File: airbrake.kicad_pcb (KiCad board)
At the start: 2 copper layers, 53.8 x 52.2 mm, 81 parts, among them IC1 SN74HCT125DR, J1 Molex Microfit, J2 Molex Microfit, J3 Molex Microfit, J4 Molex Microfit, J5 Molex Microfit, J6 Conn_02x03_Counter_Clockwise, U1 MS5607-02BA, U2 MMC5983MA, U3 STM32G431RBTx, U4 TMP275AIDGKR VSSOP8, U5 LP5912Q3.3DRVRQ1, U6 BMI088, U7 TPS62153, U8 USBLC6-2SC6, U9 W25Q256JVEIQTR, X1 1XXD32000MBA

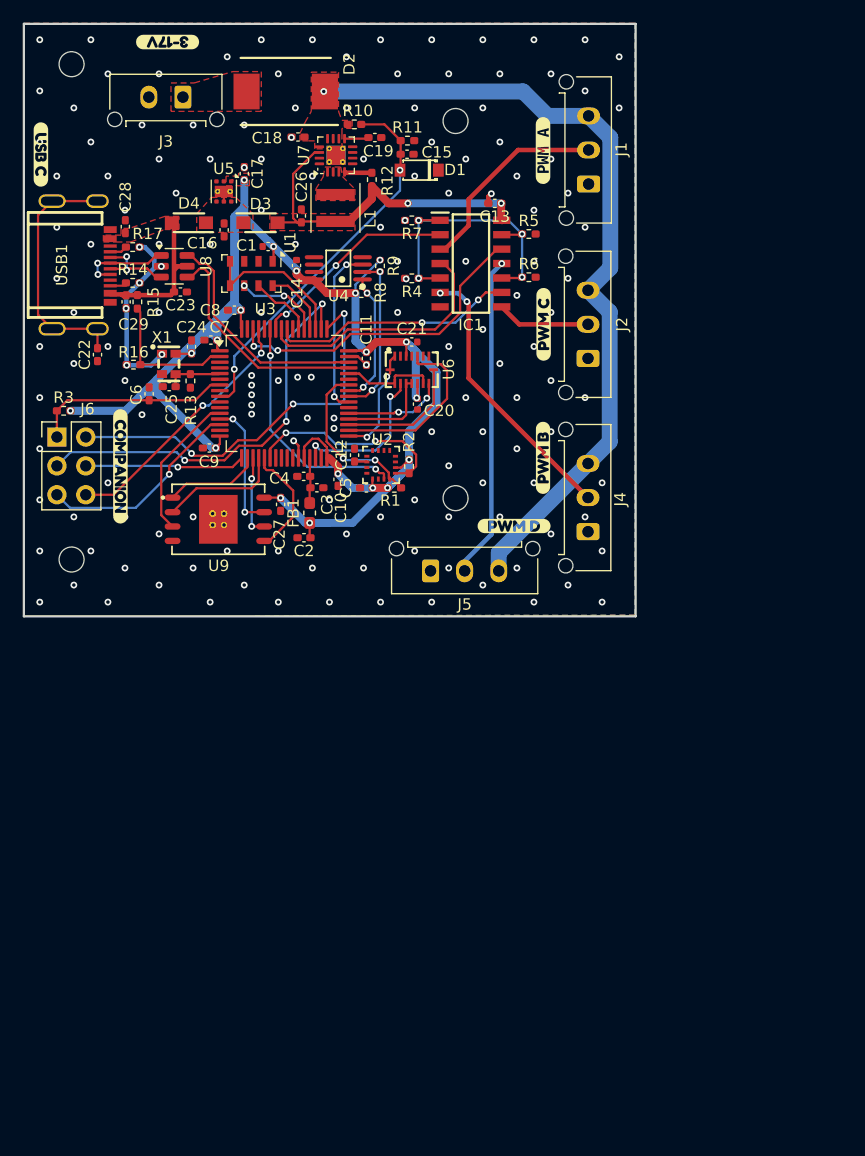
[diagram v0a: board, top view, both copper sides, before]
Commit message: release: rev1
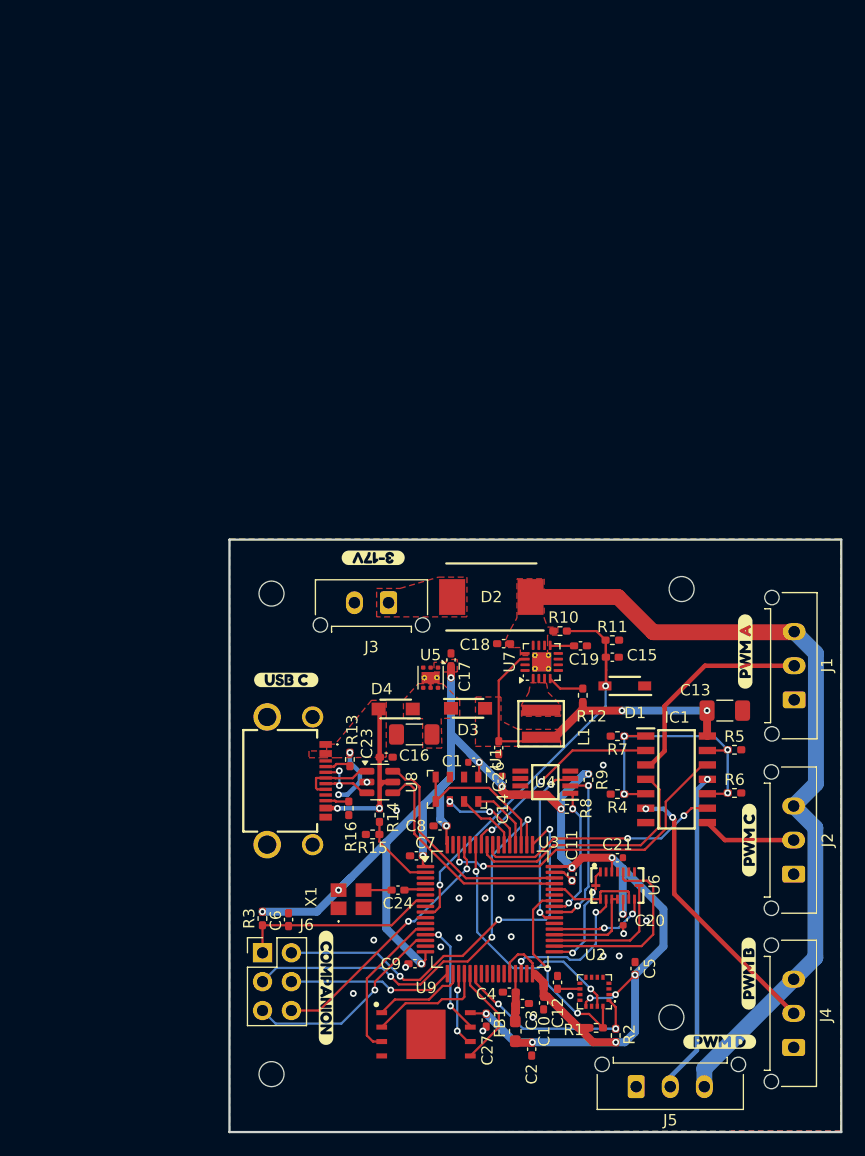
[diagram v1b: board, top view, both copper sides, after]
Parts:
- removed C22: 1nF, Capacitor_SMD:C_0402_1005Metric_Pad0.74x0.62mm_HandSolder
- removed C25: 10pF, Capacitor_SMD:C_0402_1005Metric_Pad0.74x0.62mm_HandSolder
- removed C28, C29: 10uF, Capacitor_SMD:C_0402_1005Metric_Pad0.74x0.62mm_HandSolder
- removed R17: 5.1k, Resistor_SMD:R_0402_1005Metric_Pad0.72x0.64mm_HandSolder
- removed kibuzzard-67AC9DAB: G***, kibuzzard-67AC9DAB
- added kibuzzard-67B37024: G***, kibuzzard-67B37024, F.Cu at (169.1, 89.3)
- C13, C16: footprint Capacitor_SMD:C_0402_1005Metric_Pad0.74x0.62mm_HandSolder -> Capacitor_SMD:C_1206_3216Metric_Pad1.33x1.80mm_HandSolder
- C24: value 100nF -> 10nF
- D1: footprint EasyEDA:SOD-123_L2.8-W1.8-LS3.7-RD -> SamacSys:SOD3716X135N
- D2: footprint Samacsys:DIOM7959X262N -> SamacSys:DIOM7959X262N
- D3, D4: footprint Samacsys:SODFL3616X98N -> SamacSys:SODFL3616X98N
- IC1: footprint Samacsys:SOIC127P600X175-14N -> SamacSys:SOIC127P600X175-14N
- L1: footprint Inductor_SMD:L_Coilcraft_XxL4020 -> SamacSys:XFL4020472MEC
- R13: value 100k -> 5.1k
- R14: value 5.1k -> 10k
- R15: value 10k -> 22k
- R16: value 22k -> 5.1k
- U1: value MS5607-02BA -> MS560702BA03-50
- U2: footprint EasyEDA:LGA-16_L3.0-W3.0-P0.50-BL_SQ -> SamacSys:MMC5983MA
- U4: value TMP275AIDGKR VSSOP8 -> TMP275AIDGKR; footprint EasyEDA:VSSOP-8_L3.0-W3.0-P0.65-LS5.0-BL -> SamacSys:SOP65P490X110-8N
- U9: footprint EasyEDA:WSON-8_L8.0-W6.10-P1.27-BL-EP -> SamacSys:SON127P800X600X80-9N-D
- USB1: value C169130 -> 10172013-00011LF; footprint EasyEDA:USB-C-SMD_TYPE-C3.1-02 -> SamacSys:1017201300011LF
- X1: value 1XXD32000MBA -> ECS-TXO-32CSMV-320-AN-TR; footprint EasyEDA:OSC-SMD_4P-L2.0-W1.6-BL_1XXD -> SamacSys:ECSTXO32CSMV320ANTR
- moved R2 53.3 mm to (157.7, 123.1), turned to 90 degrees
- moved R14 51.6 mm to (136.9, 103.7), turned to -90 degrees
- moved R15 51.3 mm to (136.3, 105.4), turned to 180 degrees
- moved C24 51.2 mm to (138.5, 110.3), turned to 180 degrees
- moved kibuzzard-67AC9E4A 51.0 mm to (128.7, 91.8), turned to 0 degrees
- moved R1 50.7 mm to (156.0, 122.4)
- moved U2 50.0 mm to (155.8, 119.2), turned to -90 degrees
- moved C26 49.9 mm to (147.4, 97.8), turned to 90 degrees
- moved H1 49.8 mm to (127.4, 84.2)
- moved X1 49.8 mm to (134.4, 111.1), turned to 0 degrees
- moved C12 49.7 mm to (152.6, 118.4)
- moved C10 49.5 mm to (151.3, 120.2)
- moved H4 49.5 mm to (162.6, 121.5)
- moved kibuzzard-67AC9E80 49.3 mm to (132.2, 118.9)
- moved C2 49.3 mm to (150.3, 124.3), turned to -90 degrees
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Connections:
- C24 pad 1: +3.3V -> HSE_IN
- C24 pad 2: VBAT- -> Net-(X1-OUTPUT)
- R13 pad 1: HSE_IN -> VBAT-
- R13 pad 2: VBAT- -> Net-(USB1-CC1)
- R14 pad 1: Net-(USB1-CC2) -> VBUS
- R14 pad 2: VBAT- -> BCD
- R15 pad 1: VBUS -> BCD
- R15 pad 2: BCD -> VBAT-
- R16 pad 1: BCD -> Net-(USB1-CC2)
- X1 pad 3: HSE_IN -> Net-(X1-OUTPUT)
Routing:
- net Net-(USB1-EH): track 22.0 -> 0.00 mm
- net VBAT-: track 21.9 -> 9.41 mm, vias 158 -> 22
- net BCD: track 12.0 -> 6.91 mm
- net BAT_LEVEL: track 33.6 -> 38.5 mm
- net +3.3V: track 161.6 -> 166.0 mm
- net +3.3VA: track 3.86 -> 7.29 mm
- net HSE_IN: track 4.94 -> 1.88 mm
- net MMC5983MA_SDA: track 15.0 -> 17.7 mm
- net Net-(X1-OUTPUT): track 0.00 -> 2.47 mm
- net VBUS: track 15.8 -> 17.6 mm, vias 0 -> 2
- net +5V: track 30.3 -> 32.1 mm
- net D+: track 7.51 -> 6.02 mm, vias 2 -> 0
- net BMI088_GYRO_CS: track 15.8 -> 16.9 mm
- net MMC5983MA_INT: track 21.0 -> 22.0 mm
- net W25Q_HOLD: track 11.5 -> 10.4 mm
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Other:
- board size 53.8 x 52.2 mm -> 53.9 x 52.1 mm
